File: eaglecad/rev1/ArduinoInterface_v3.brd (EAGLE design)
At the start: 141.9 x 73.6 mm, 49 parts, among them IC1 74LS00N, IC10 74LS241N, IC11 74LS20N, IC3 74LS30N, IC5 74S74N, IC6 74LS139N, IC7 74LS155N, IC8 74LS241N, IC9 7805TV, J1 Connector, J2 TEENSY_CONN, J3 GLUE_CONN

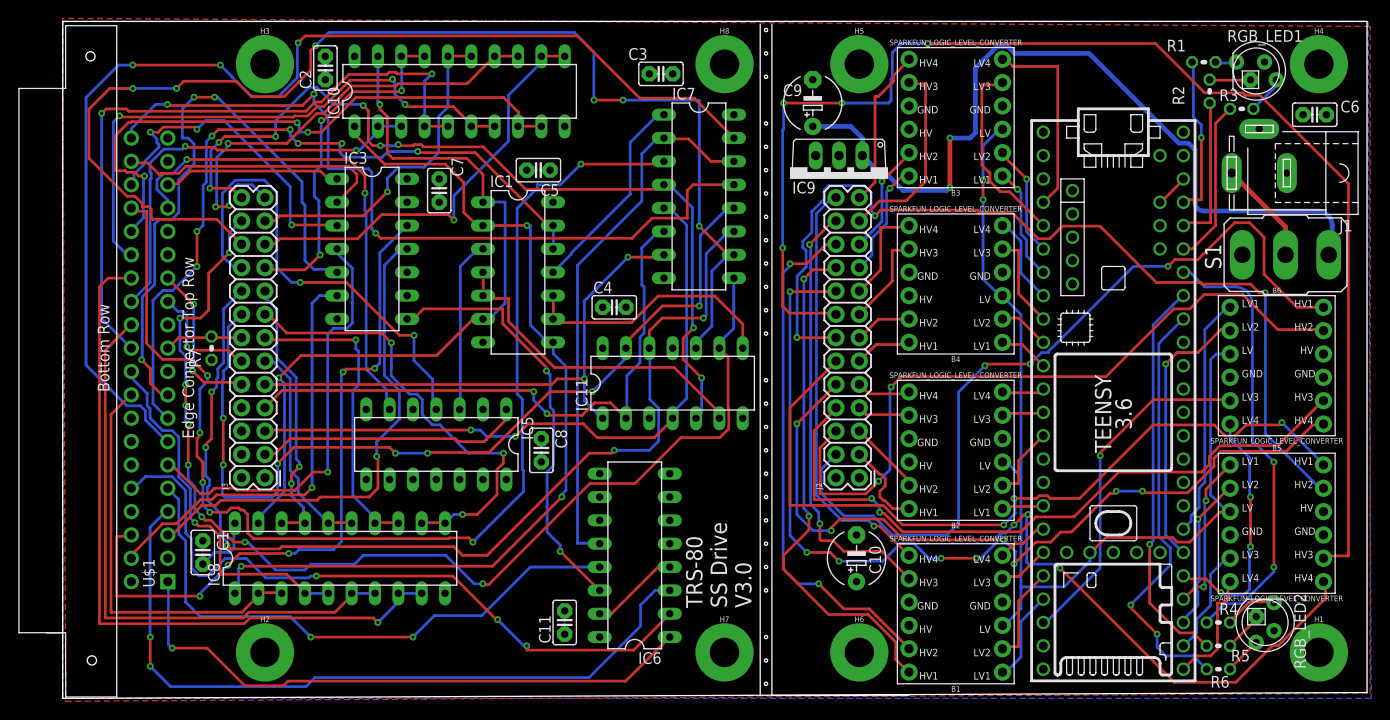
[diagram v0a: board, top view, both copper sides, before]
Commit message: updated schematic to fix 74LS241/74LS244 mixup
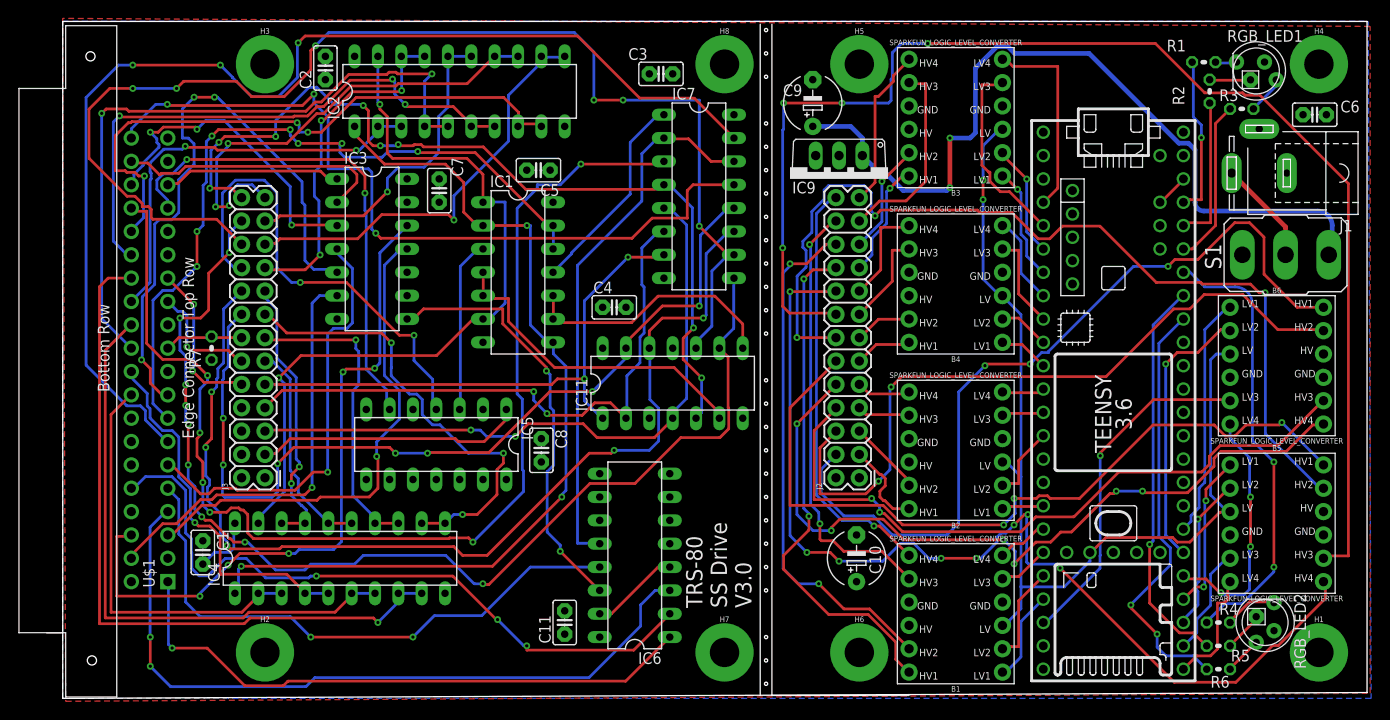
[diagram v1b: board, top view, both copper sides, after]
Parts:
- IC2, IC4: value 74LS241N -> 74LS244N
- renumbered IC10 to IC2, IC8 to IC4
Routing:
- net D2_HV: track 46.5 -> 47.7 mm
- net D3: track 45.9 -> 46.9 mm

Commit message: updating schematics
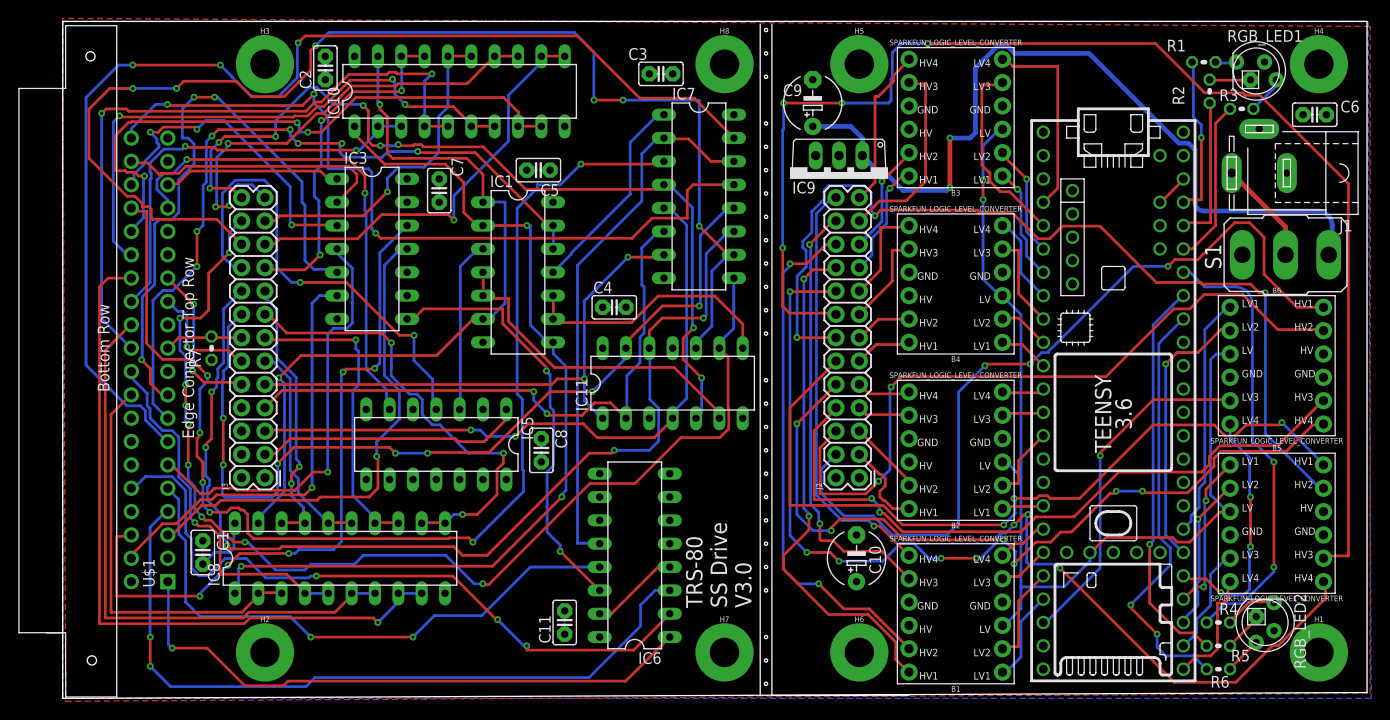
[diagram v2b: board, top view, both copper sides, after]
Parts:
- IC10, IC8: value 74LS244N -> 74LS241N
- renumbered IC2 to IC10, IC4 to IC8
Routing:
- net D2_HV: track 47.7 -> 46.5 mm
- net D3: track 46.9 -> 45.9 mm
